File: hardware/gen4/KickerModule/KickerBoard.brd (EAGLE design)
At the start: 328.9 x 149.3 mm, 119 parts

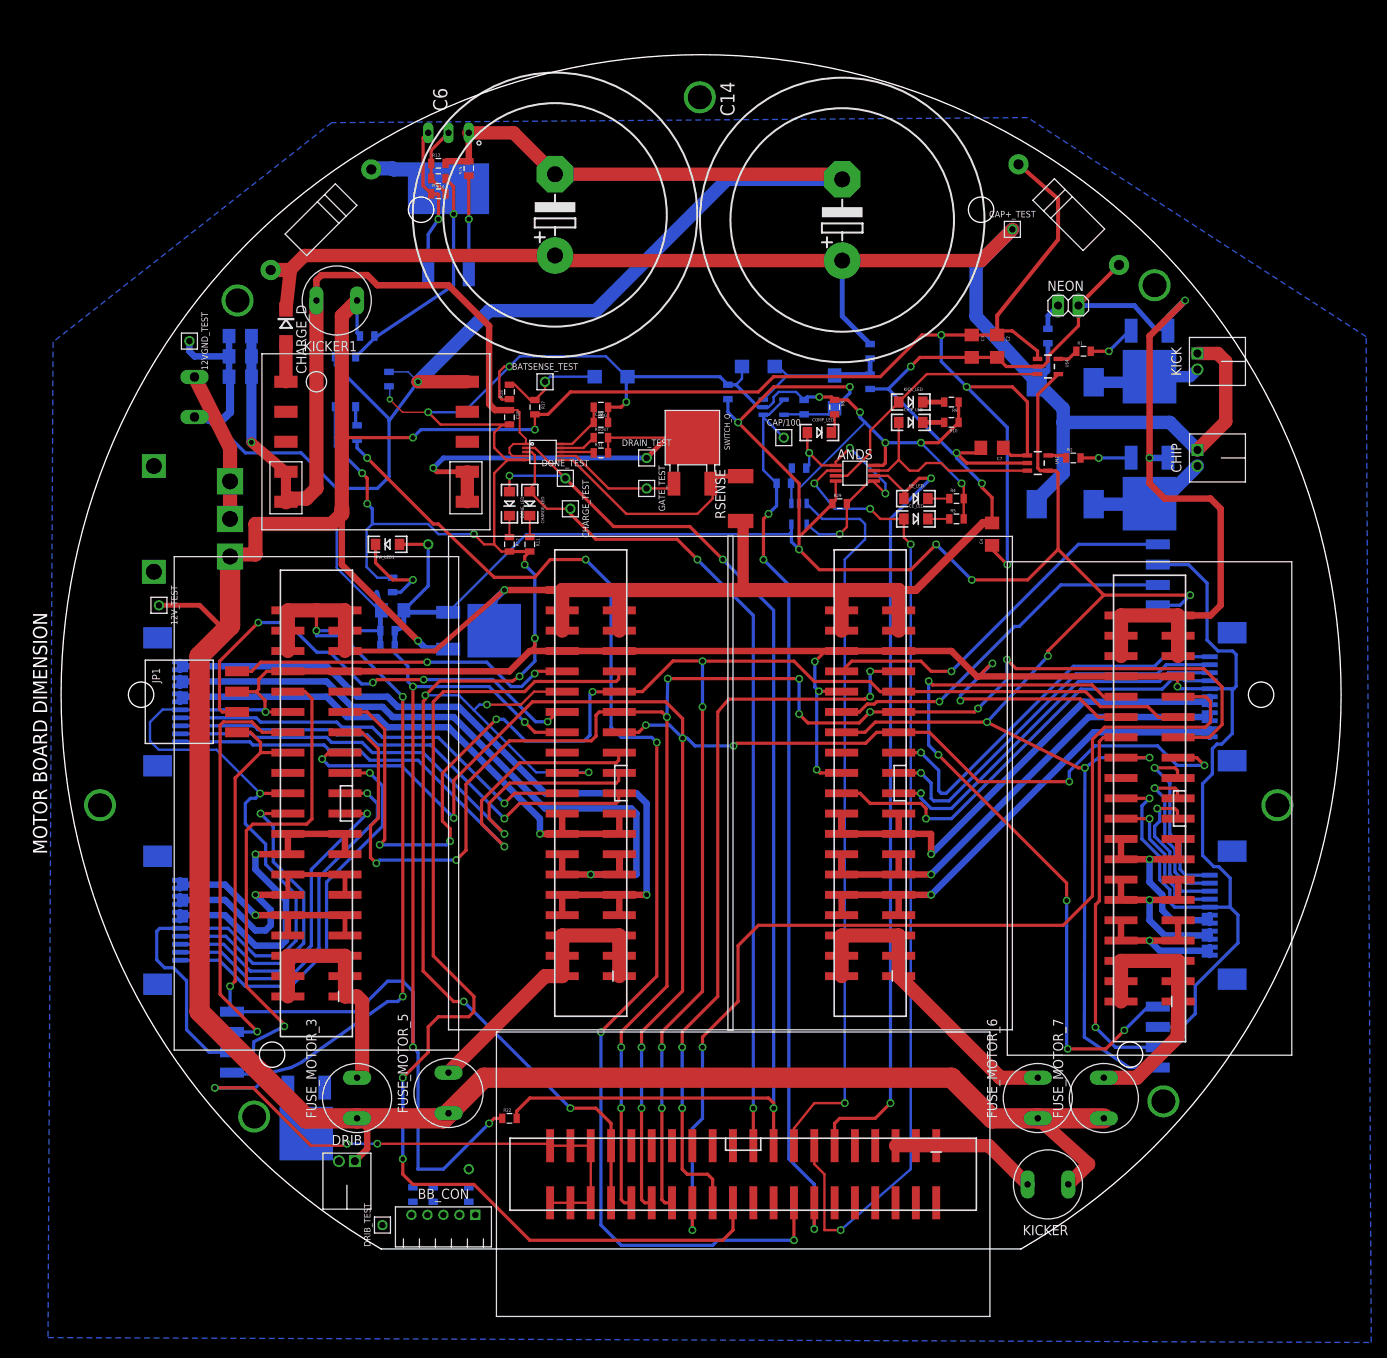
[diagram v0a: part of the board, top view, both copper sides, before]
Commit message: moving things around
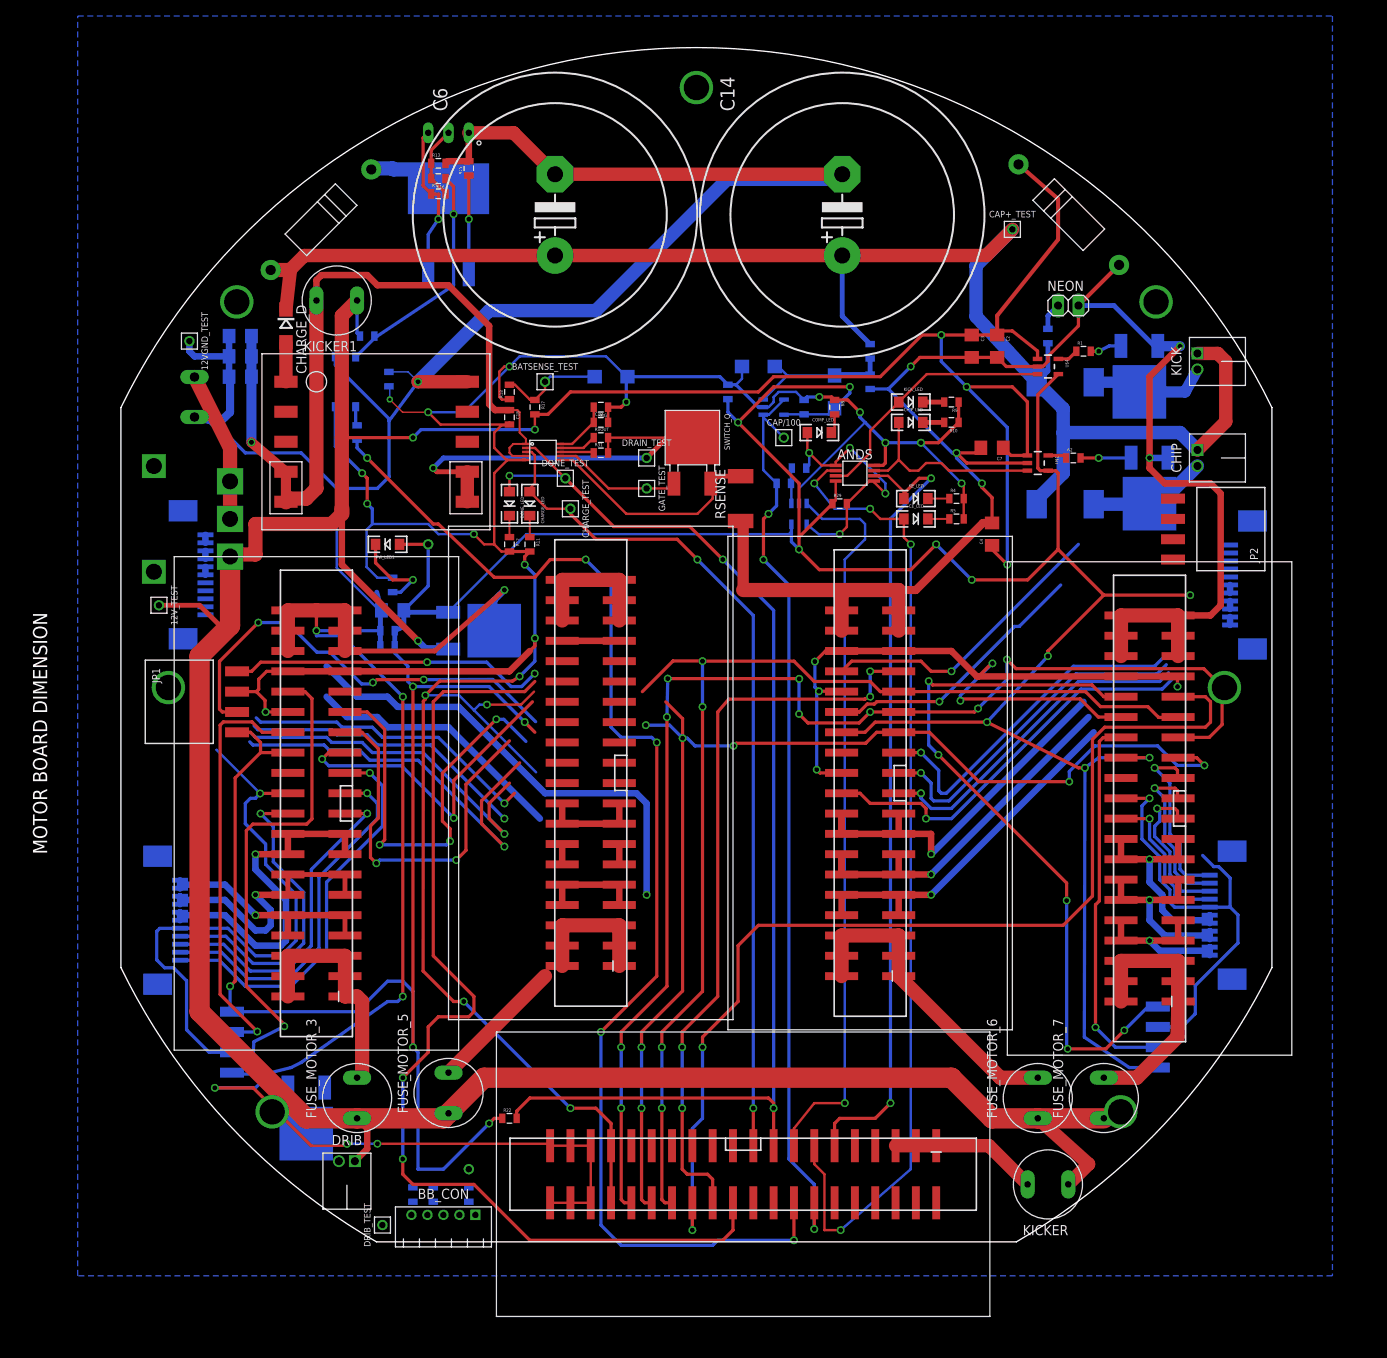
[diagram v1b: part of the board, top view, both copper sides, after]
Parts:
- moved U$8 16.2 mm to (6.35, 90.8)
- moved U$9 14.2 mm to (138.4, 89.5)
- moved JP2 6.02 mm to (136.5, 96.5), flipped to the top, turned to 90 degrees
- moved KICK_Q 2.29 mm to (125.1, 113.7)
- moved MOTOR2 1.27 mm to (56.5, 66.0)
- moved C14 0.63 mm to (88.0, 135.8)
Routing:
- net GND: track 755.3 -> 630.7 mm, vias 29 -> 28
- net N$38: track 93.9 -> 6.08 mm, vias 1 -> 0
- net 12VGND: track 684.0 -> 653.0 mm
- net N$43: track 61.5 -> 36.1 mm
- net N$44: track 68.7 -> 44.9 mm
- net N$39: track 69.8 -> 46.2 mm, vias 1 -> 0
- net MISO: track 231.0 -> 208.1 mm
- net N$45: track 73.1 -> 50.9 mm
- net N$37: track 93.8 -> 71.8 mm
- net MOSI: track 209.8 -> 189.4 mm
- net SCK: track 215.3 -> 195.2 mm, vias 8 -> 7
- net N$56: track 65.8 -> 49.6 mm
- net N$55: track 63.6 -> 48.0 mm
- net N$42: track 52.7 -> 37.2 mm
- net N$54: track 61.1 -> 46.0 mm
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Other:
- board size 328.9 x 149.3 mm -> 320.2 x 149.3 mm
